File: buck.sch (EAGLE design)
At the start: 30 parts, among them J1 B06B-HCMKK, J2 POWERPOLE_POWER45A_DRILL, J3 POWERPOLE_POWER45A_DRILL

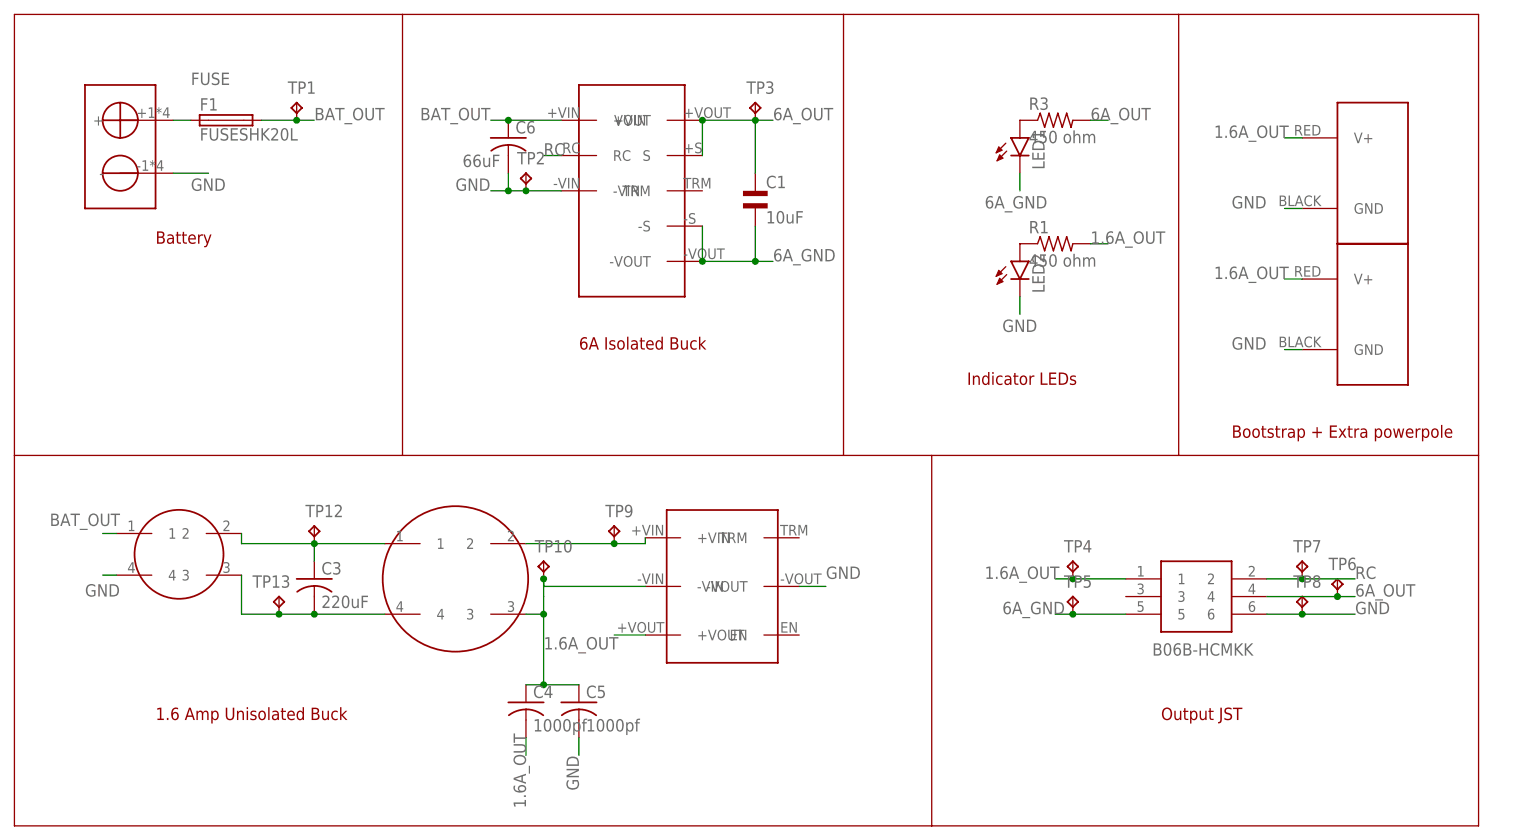
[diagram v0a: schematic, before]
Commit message: Add files via upload
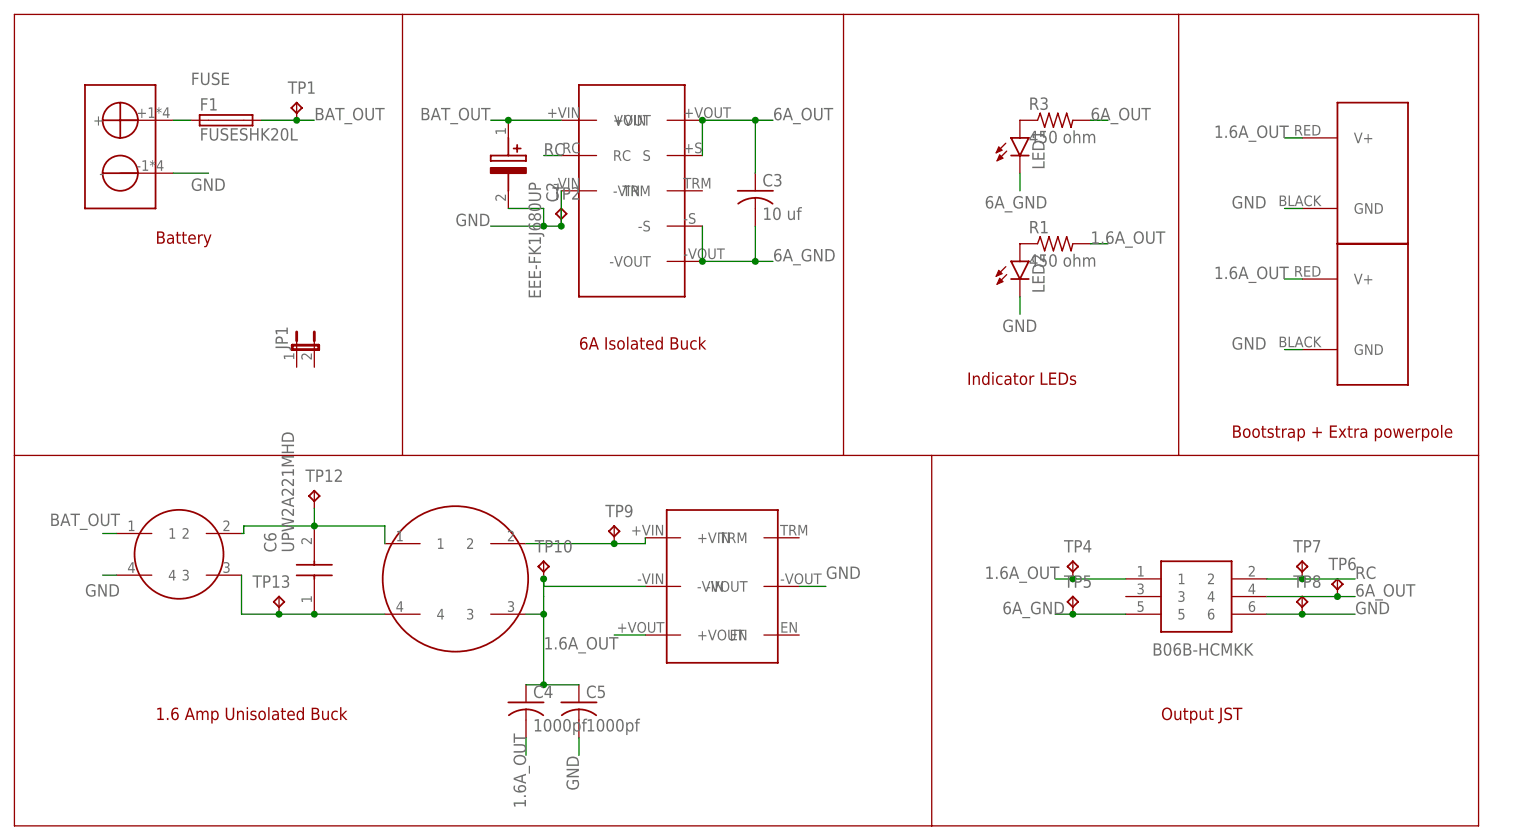
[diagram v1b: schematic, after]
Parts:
- removed C1: 10uF, rcl:EL-BI25-10AXIAL
- removed TP3: TPPAD1-13, testpad:TPPAD1-13
- added C2: EEE-FK1J680UP, SamacSys_Parts:EEE-FK1J680UP
- added JP1: (no value), jumper:JP1E
- C3: value 220uF -> 10 uf
- C6: value 66uF -> UPW2A221MHD; device rcl:C-USC0805 -> SamacSys_Parts:UPW2A221MHD
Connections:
- removed net N$3: BUCK150UH.2, C3.1, CHOKEME.1, TP12.TP
- new net N$1: BUCK150UH.2, C6.-, CHOKEME.1, TP12.TP
- net 6A_GND: now also C3.2; no longer C1.2
- net 6A_OUT: now also C3.1; no longer C1.1, TP3.TP
- net BAT_OUT: now also C2.+; no longer C6.1
- net GND: now also C2.-; no longer C6.2
- net N$4: now also C6.+; no longer C3.2
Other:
- moved on the sheet: C3, TP12, TP2
